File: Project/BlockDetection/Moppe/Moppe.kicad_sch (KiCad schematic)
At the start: 10 parts, among them J1 Conn_01x03_Pin, J2 Conn_01x02_Pin, Q1 BC856 or BC557, U1 PC817

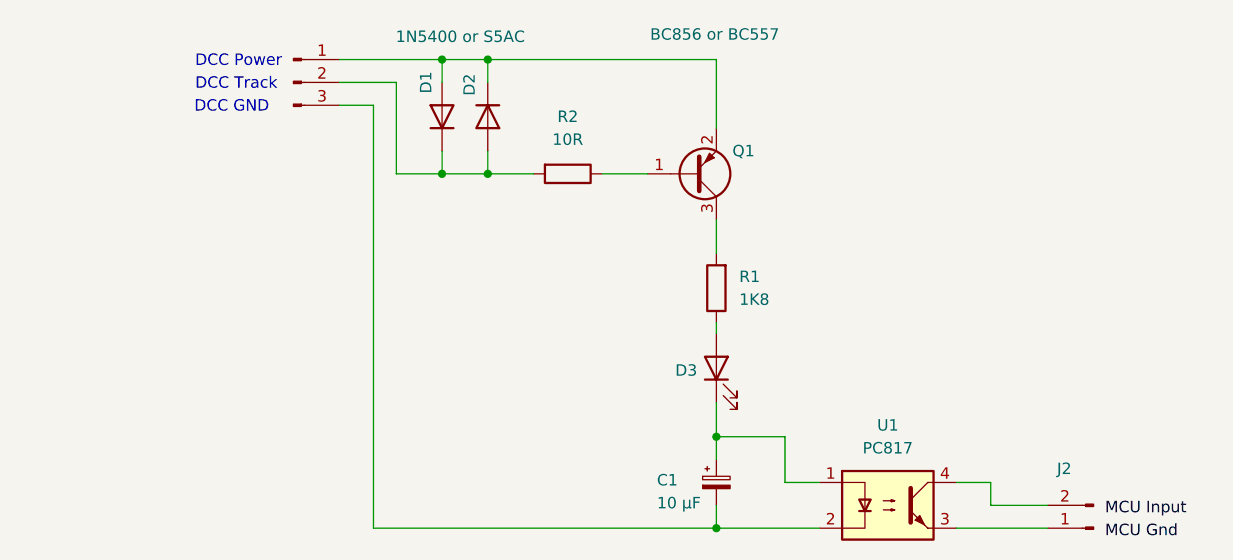
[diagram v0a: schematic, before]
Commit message: SporBesat a la´ Moppe
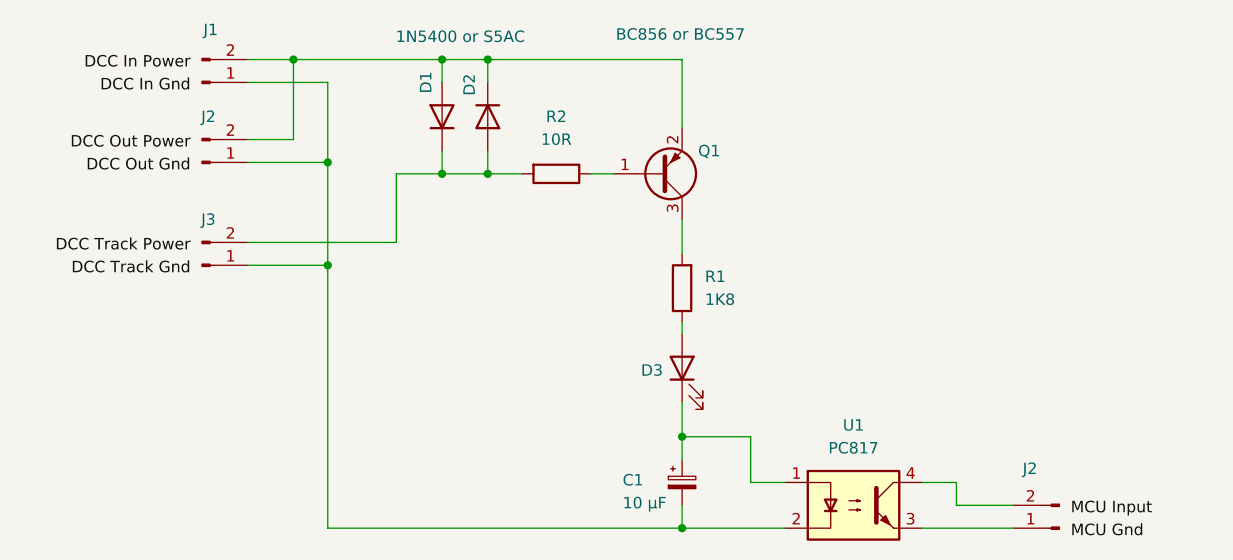
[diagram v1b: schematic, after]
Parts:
- removed J1: Conn_01x03_Pin, symbol Connector:Conn_01x03_Pin
- added J1, J2, J3: Conn_01x02_Pin, Connector:Tag-Connect_TC2030-IDC-FP_2x03_P1.27mm_Vertical, symbol Connector:Conn_01x02_Pin
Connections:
- net at C1.2, U1.2: now also J1.1 (Pin_1), J2.1 (Pin_1), J3.1 (Pin_1)
- net at D1.2 (A), D2.1 (K), Q1.2 (E): now also J1.2 (Pin_2), J2.2 (Pin_2)
- net at D1.1 (K), D2.2 (A), R2.2: now also J3.2 (Pin_2)
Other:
- note removed: "DCC GND"
- note removed: "DCC Power"
- note removed: "DCC Track"
- moved on the sheet: C1, D3, J2, Q1, R1, R2, U1

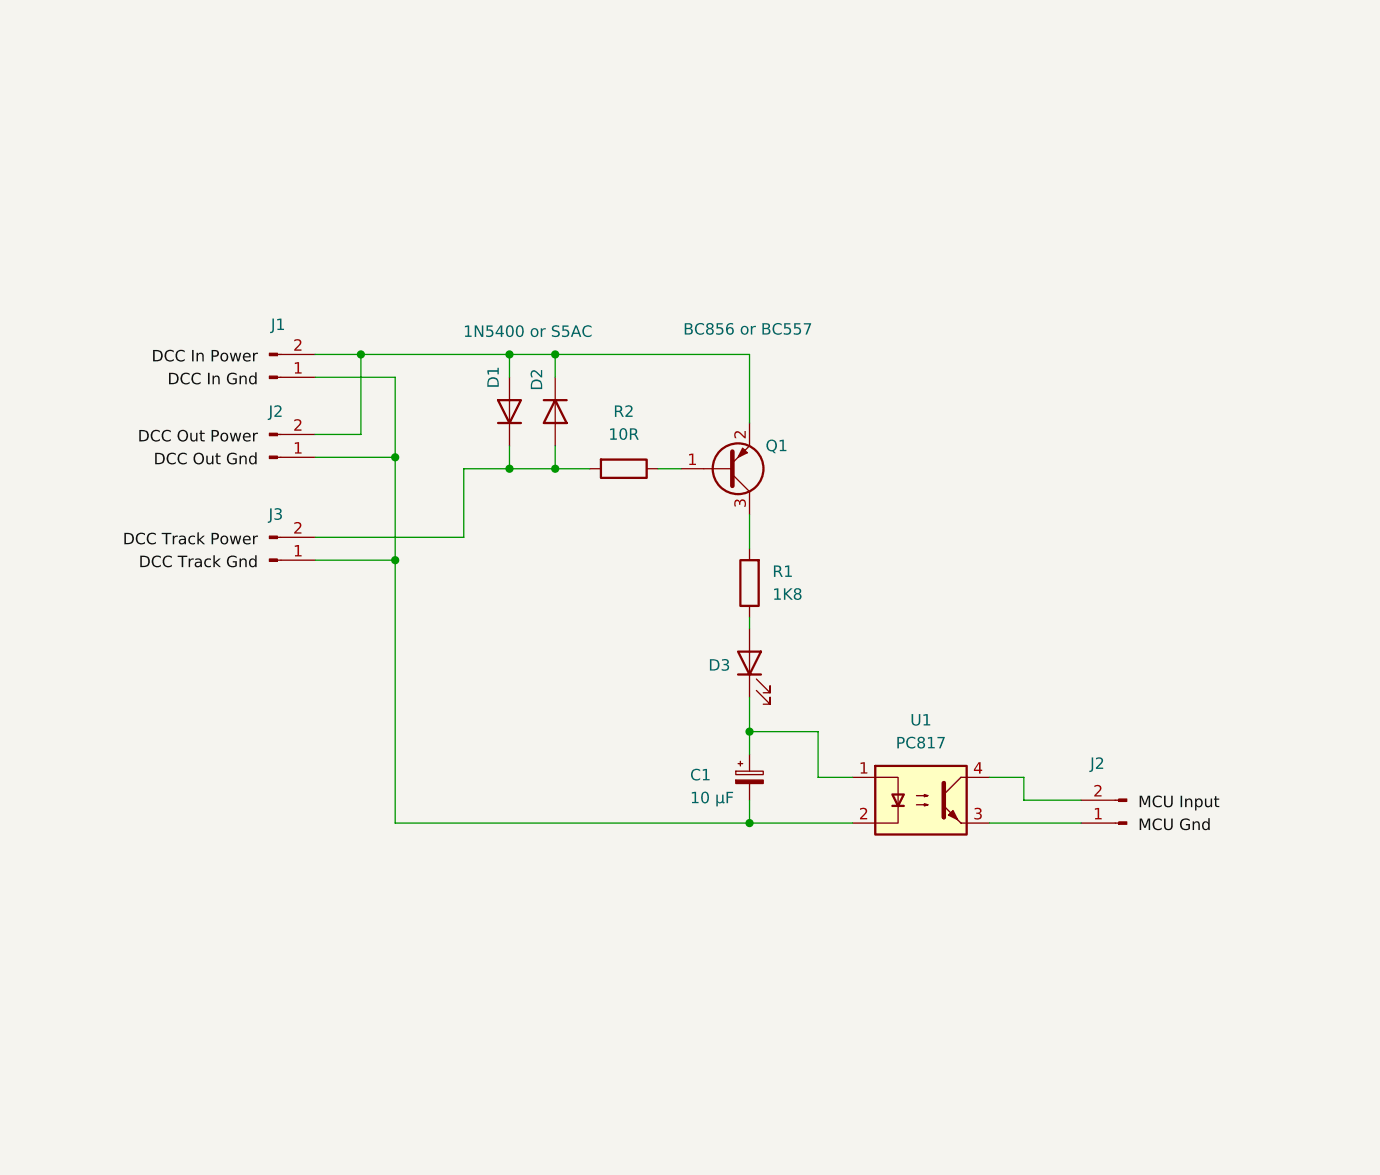
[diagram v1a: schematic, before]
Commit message: SporBesat a la´ Moppe
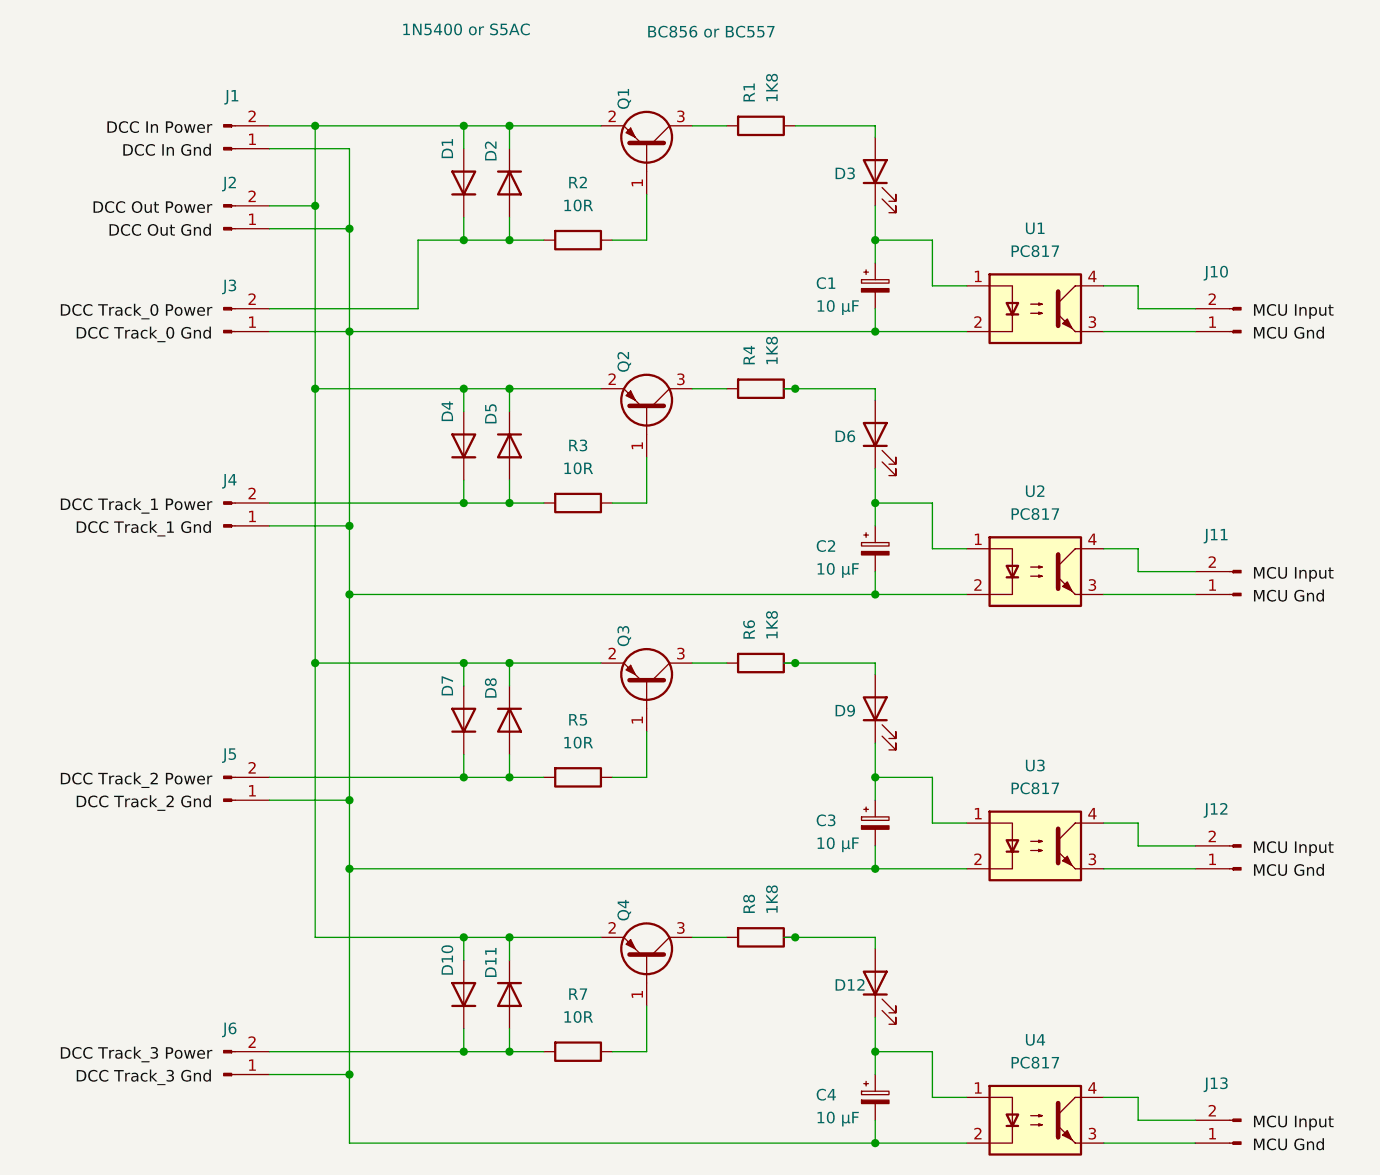
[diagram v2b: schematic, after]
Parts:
- added C2, C3, C4: 10 µF, symbol Device:C_Polarized_Small
- added D10, D4, D7: 1N5400 or S5AC, Diode_THT:D_DO-201AD_P15.24mm_Horizontal, symbol Diode:1N5400
- added D11, D5, D8: 1N5400, Diode_THT:D_DO-201AD_P15.24mm_Horizontal, symbol Diode:1N5400
- added D12, D6, D9: IR26-21C_L110_TR8, LED_SMD:LED_1206_3216Metric, symbol LED:IR26-21C_L110_TR8
- added J11, J12, J13, J4, J5, J6: Conn_01x02_Pin, Connector:Tag-Connect_TC2030-IDC-FP_2x03_P1.27mm_Vertical, symbol Connector:Conn_01x02_Pin
- added Q2, Q3, Q4: BC856 or BC557, Package_TO_SOT_SMD:SOT-23, symbol Transistor_BJT:BC856
- added R3, R5, R7: 10R, symbol Device:R
- added R4, R6, R8: 1K8, symbol Device:R
- added U2, U3, U4: PC817, Package_DIP:DIP-4_W7.62mm, symbol Isolator:PC817
- renumbered J2 to J10
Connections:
- net at C1.2, J1.1 (Pin_1), J2.1 (Pin_1)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: now also C2.2, C3.2, C4.2, J4.1 (Pin_1), J5.1 (Pin_1), J6.1 (Pin_1), U2.2, U3.2, U4.2
- net at D1.2 (A), D2.1 (K), J1.2 (Pin_2)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: now also D10.2 (A), D11.1 (K), D4.2 (A), D5.1 (K), D7.2 (A), D8.1 (K), Q2.2 (E), Q3.2 (E), Q4.2 (E)
- new net: D4.1 (K), D5.2 (A), J4.2 (Pin_2), R3.2
- new net: C4.1, D12.1 (K), U4.1
- new net: J12.1 (Pin_1), U3.3
- new net: J12.2 (Pin_2), U3.4
- new net: D6.2 (A), R4.1
- new net: Q2.3 (C), R4.2
- new net: Q2.1 (B), R3.1
- new net: C2.1, D6.1 (K), U2.1
- new net: D7.1 (K), D8.2 (A), J5.2 (Pin_2), R5.2
- new net: D9.2 (A), R6.1
- new net: Q3.3 (C), R6.2
- new net: J11.1 (Pin_1), U2.3
- new net: J11.2 (Pin_2), U2.4
- new net: D12.2 (A), R8.1
- new net: C3.1, D9.1 (K), U3.1
- new net: Q3.1 (B), R5.1
- new net: Q4.1 (B), R7.1
- new net: D10.1 (K), D11.2 (A), J6.2 (Pin_2), R7.2
- new net: Q4.3 (C), R8.2
- new net: J13.1 (Pin_1), U4.3
- new net: J13.2 (Pin_2), U4.4
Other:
- moved on the sheet: C1, D1, D2, D3, J1, J10, J2, J3, Q1, R1, R2, U1
